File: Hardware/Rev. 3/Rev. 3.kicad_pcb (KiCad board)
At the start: 4 copper layers, 23.4 x 23.4 mm, 16 parts, among them J1 84952-8, Q1 NMOS, U1 MCP73831-2-OT, U3 W25Q128JVS

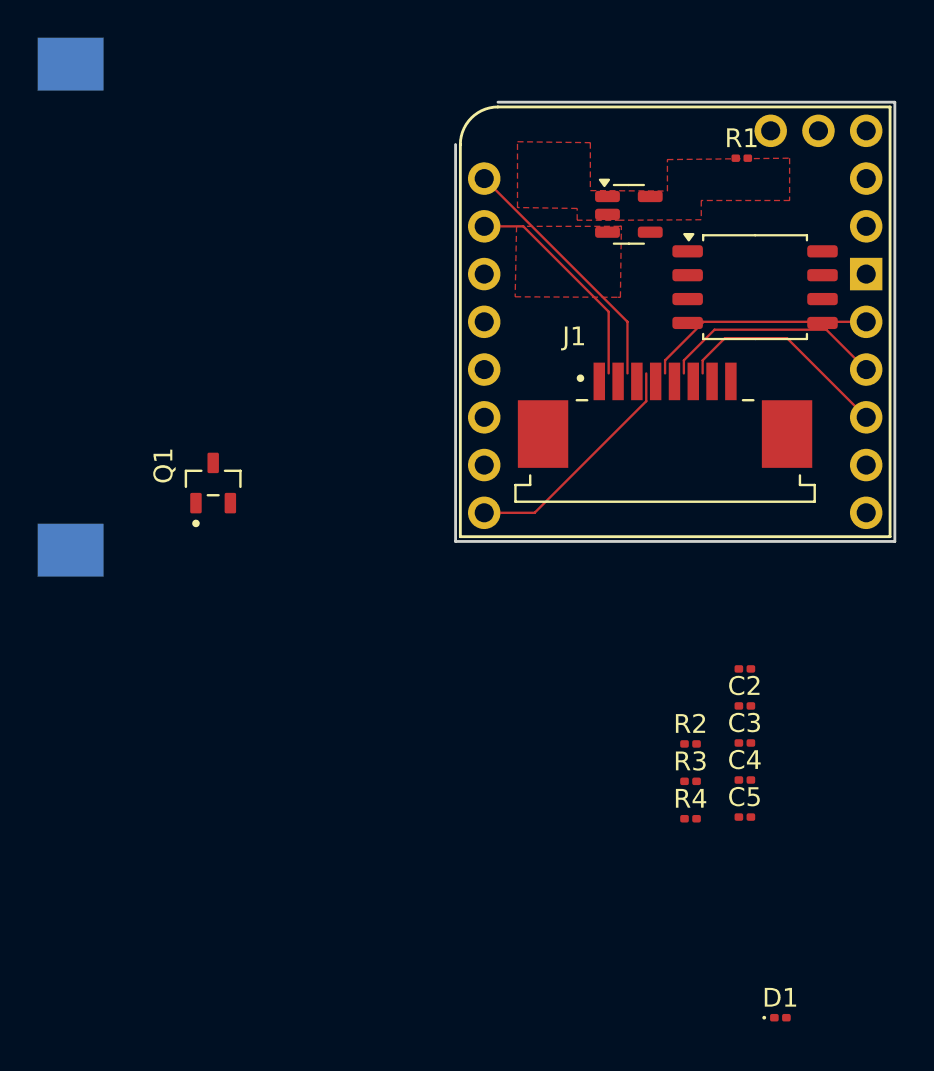
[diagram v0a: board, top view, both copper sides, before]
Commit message: Week 13 Changes
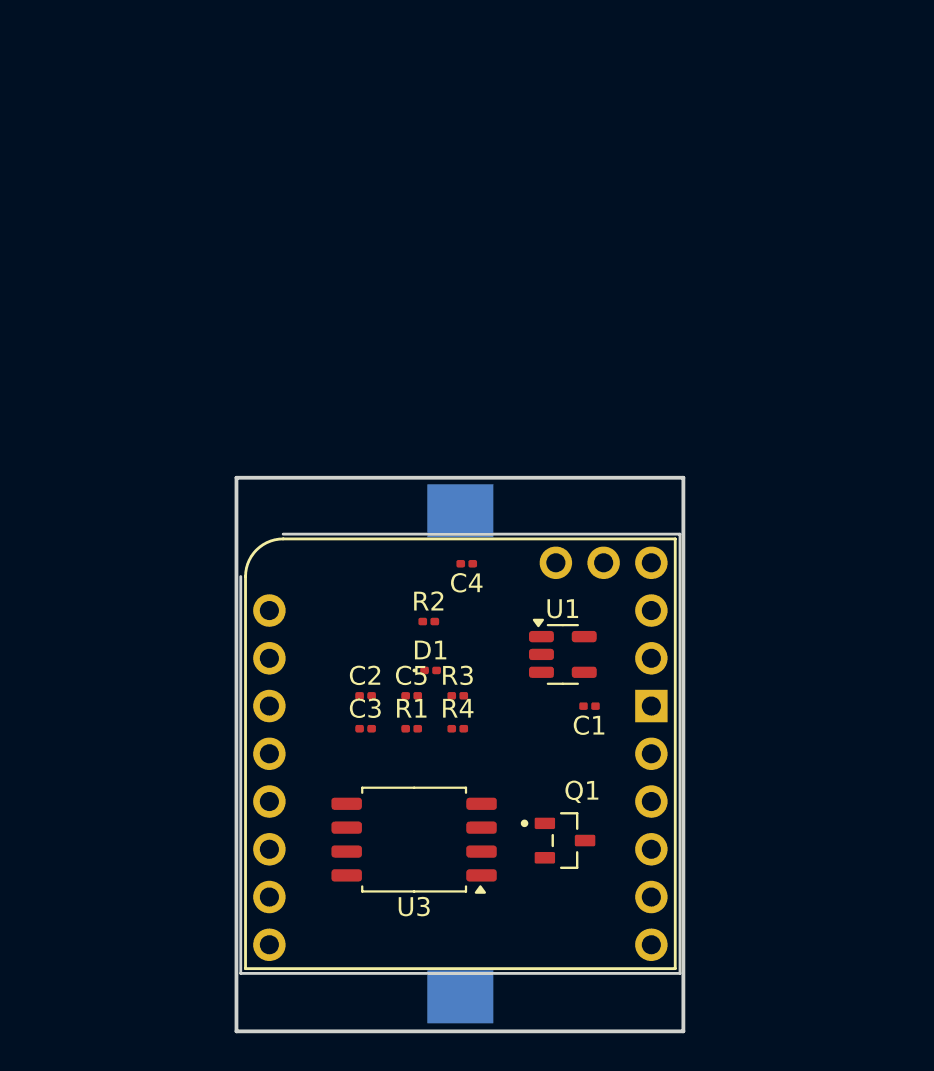
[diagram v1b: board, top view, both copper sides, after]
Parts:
- removed J1: 84952-8, footprints:FFC_84952-8
- moved R1 35.1 mm to (165.5, 96.7)
- moved U3 34.5 mm to (165.7, 102.6), turned to 180 degrees
- moved BT1 31.5 mm to (168.1, 98.0), turned to 90 degrees
- moved Q1 26.7 mm to (173.7, 102.7), turned to 0 degrees
- moved D1 26.2 mm to (166.5, 93.6)
- moved U2 25.7 mm to (156.7, 86.6)
- moved U1 23.7 mm to (173.6, 92.8)
- moved C3 20.2 mm to (163.1, 96.7)
- moved C2 20.2 mm to (163.1, 95.0)
- moved C5 18.9 mm to (165.5, 95.0)
- moved C4 18.7 mm to (168.4, 87.9), turned to 180 degrees
- moved R2 15.4 mm to (166.4, 91.0)
- moved R4 13.3 mm to (168.0, 96.7)
- moved R3 13.2 mm to (168.0, 95.0)
- moved C1 8.50 mm to (175.0, 95.5), turned to 180 degrees
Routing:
- net 10/A0: track 13.5 -> 0.00 mm
- net 5/LPIO0: track 12.6 -> 0.00 mm
- net 0/LPIO3: track 12.2 -> 0.00 mm
- net 1/LPIO2/RX: track 11.9 -> 0.00 mm
- net 11/A1: track 11.8 -> 0.00 mm
- net 2/LPIO1/TX: track 11.6 -> 0.00 mm
- removed copper zone on F.Cu, net GND
- removed copper zone on F.Cu, net VBAT
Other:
- board size 23.4 x 23.4 mm -> 23.8 x 29.5 mm
